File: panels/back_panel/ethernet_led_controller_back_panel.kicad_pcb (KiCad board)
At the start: 2 copper layers, 60 x 100 mm, 0 parts

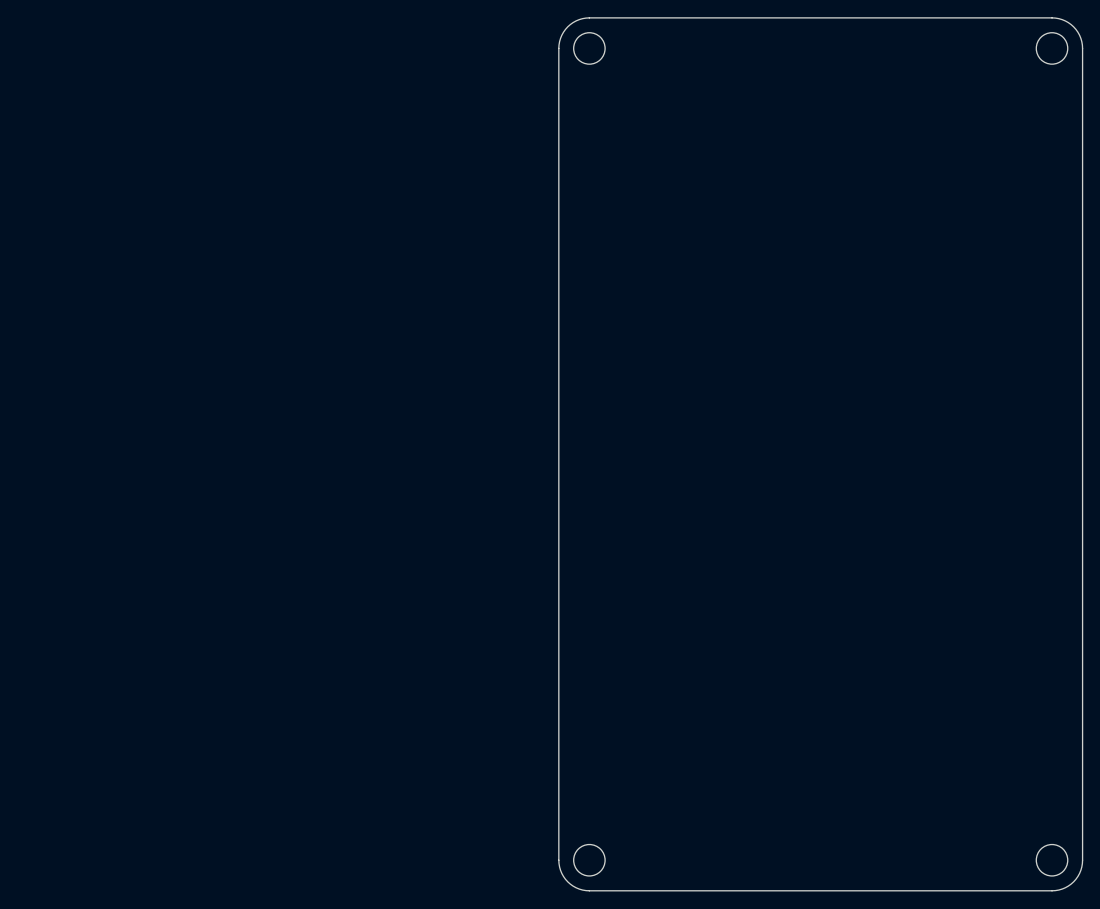
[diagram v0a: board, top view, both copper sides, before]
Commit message: update hardware to v1_2_0
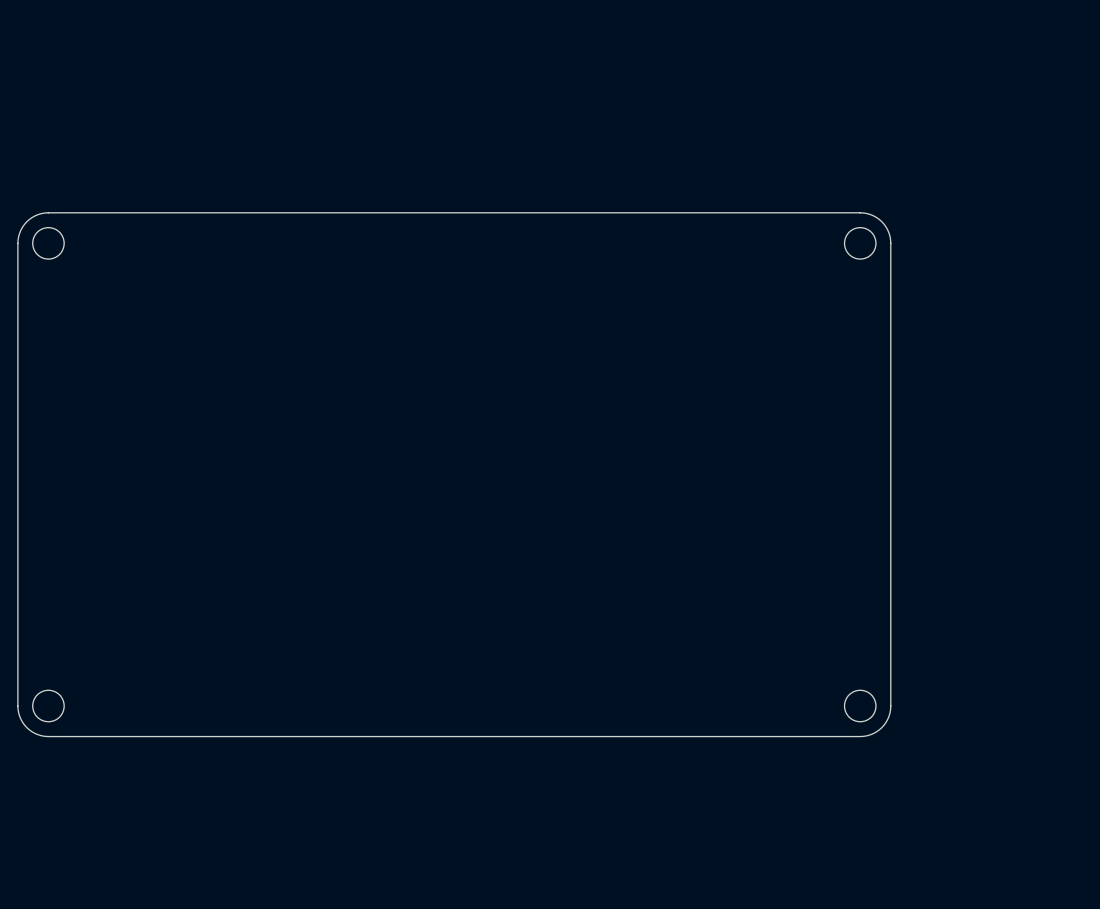
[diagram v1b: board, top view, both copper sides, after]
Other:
- board size 60 x 100 mm -> 100 x 60 mm
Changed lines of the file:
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@@
   )
   (net 0 "")
-  (gr_line (start 210.87 130.17) (end 157.87 130.17)
+  (gr_line (start 192.4 56) (end 192.4 109)
     (stroke (width 0.1) (type default)) (layer "Edge.Cuts"))
-  (gr_line (start 154.37 126.67) (end 154.37 33.67)
+  (gr_line (start 188.9 112.5) (end 95.9 112.5)
     (stroke (width 0.1) (type default)) (layer "Edge.Cuts"))
-  (gr_circle (center 157.87 126.67) (end 157.87 124.87)
+  (gr_circle (center 188.9 109) (end 187.1 109)
     (stroke (width 0.1) (type default)) (fill none) (layer "Edge.Cuts"))
-  (gr_line (start 157.87 30.17) (end 210.87 30.17)
+  (gr_line (start 92.4 109) (end 92.4 56)
     (stroke (width 0.1) (type default)) (layer "Edge.Cuts"))
-  (gr_circle (center 210.87 33.67) (end 210.87 35.47)
+  (gr_circle (center 95.9 56) (end 97.7 56)
     (stroke (width 0.1) (type default)) (fill none) (layer "Edge.Cuts"))
-  (gr_arc (start 210.87 30.17) (mid 213.344874 31.195126) (end 214.37 33.67)
+  (gr_arc (start 92.4 56) (mid 93.425126 53.525126) (end 95.9 52.5)
     (stroke (width 0.1) (type default)) (layer "Edge.Cuts"))
-  (gr_arc (start 157.87 130.17) (mid 155.395126 129.144874) (end 154.37 126.67)
+  (gr_arc (start 192.4 109) (mid 191.374874 111.474874) (end 188.9 112.5)
     (stroke (width 0.1) (type default)) (layer "Edge.Cuts"))
-  (gr_circle (center 210.87 126.67) (end 210.87 124.87)
+  (gr_circle (center 188.9 56) (end 187.1 56)
     (stroke (width 0.1) (type default)) (fill none) (layer "Edge.Cuts"))
-  (gr_circle (center 157.87 33.67) (end 157.87 35.47)
+  (gr_circle (center 95.9 109) (end 97.7 109)
     (stroke (width 0.1) (type default)) (fill none) (layer "Edge.Cuts"))
-  (gr_arc (start 214.37 126.67) (mid 213.344874 129.144874) (end 210.87 130.17)
+  (gr_arc (start 188.9 52.5) (mid 191.374874 53.525126) (end 192.4 56)
     (stroke (width 0.1) (type default)) (layer "Edge.Cuts"))
-  (gr_arc (start 154.37 33.67) (mid 155.395126 31.195126) (end 157.87 30.17)
+  (gr_arc (start 95.9 112.5) (mid 93.425126 111.474874) (end 92.4 109)
     (stroke (width 0.1) (type default)) (layer "Edge.Cuts"))
-  (gr_line (start 214.37 33.67) (end 214.37 126.67)
+  (gr_line (start 95.9 52.5) (end 188.9 52.5)
     (stroke (width 0.1) (type default)) (layer "Edge.Cuts"))
-  (gr_text "JLCJLCJLCJLC" (at 207.17 129.37) (layer "B.SilkS")
+  (gr_text "JLCJLCJLCJLC" (at 191.6 59.7 90) (layer "B.SilkS")
     (effects (font (size 0.81 0.81) (thickness 0.04)) (justify mirror))
   )
